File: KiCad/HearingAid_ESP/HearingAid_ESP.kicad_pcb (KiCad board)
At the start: 2 copper layers, 69.2 x 22.1 mm, 63 parts, among them J1 12402012E212A, Q1 PMOS, Q2 FS8205A, U1 AP2112K-3.3, U2 MAX98357A, U3 TP4056, U4 DW01A, U5 MAX98357A, U8 ESP32-S3

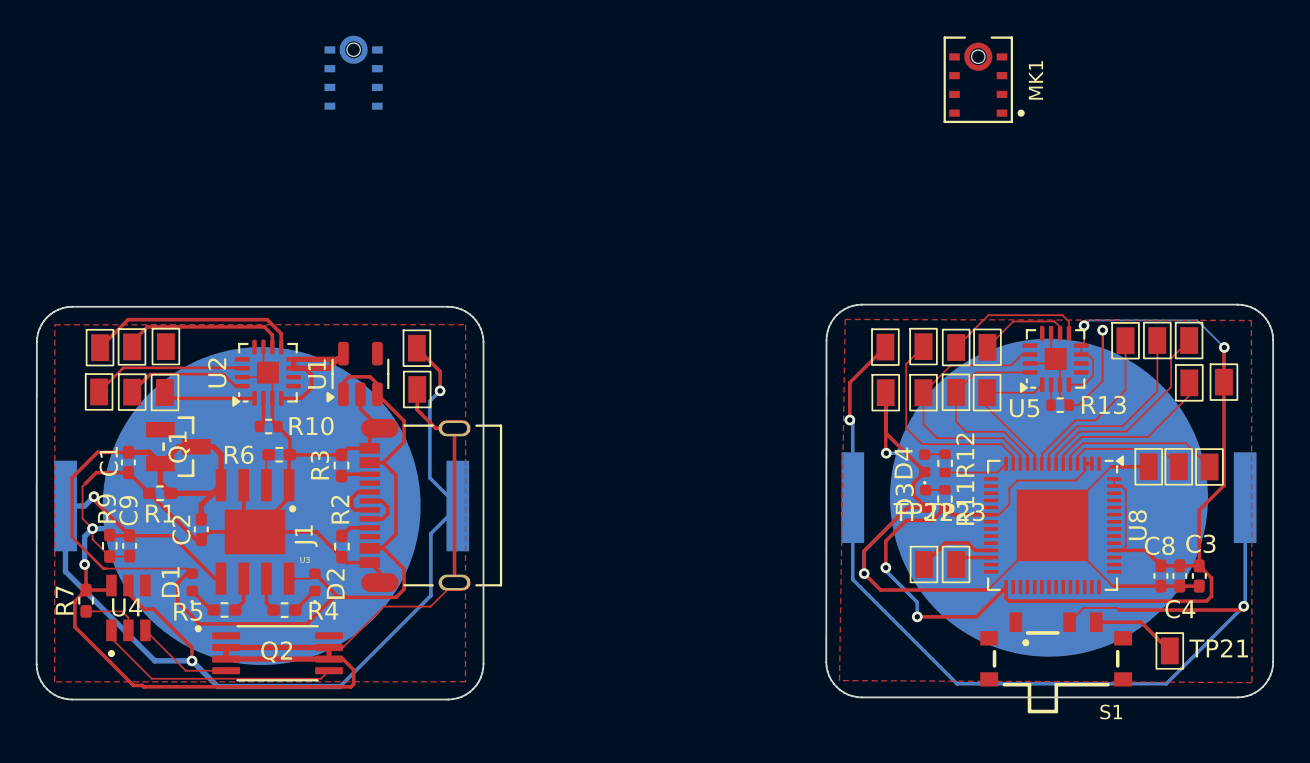
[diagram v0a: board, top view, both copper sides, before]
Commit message: Updating files
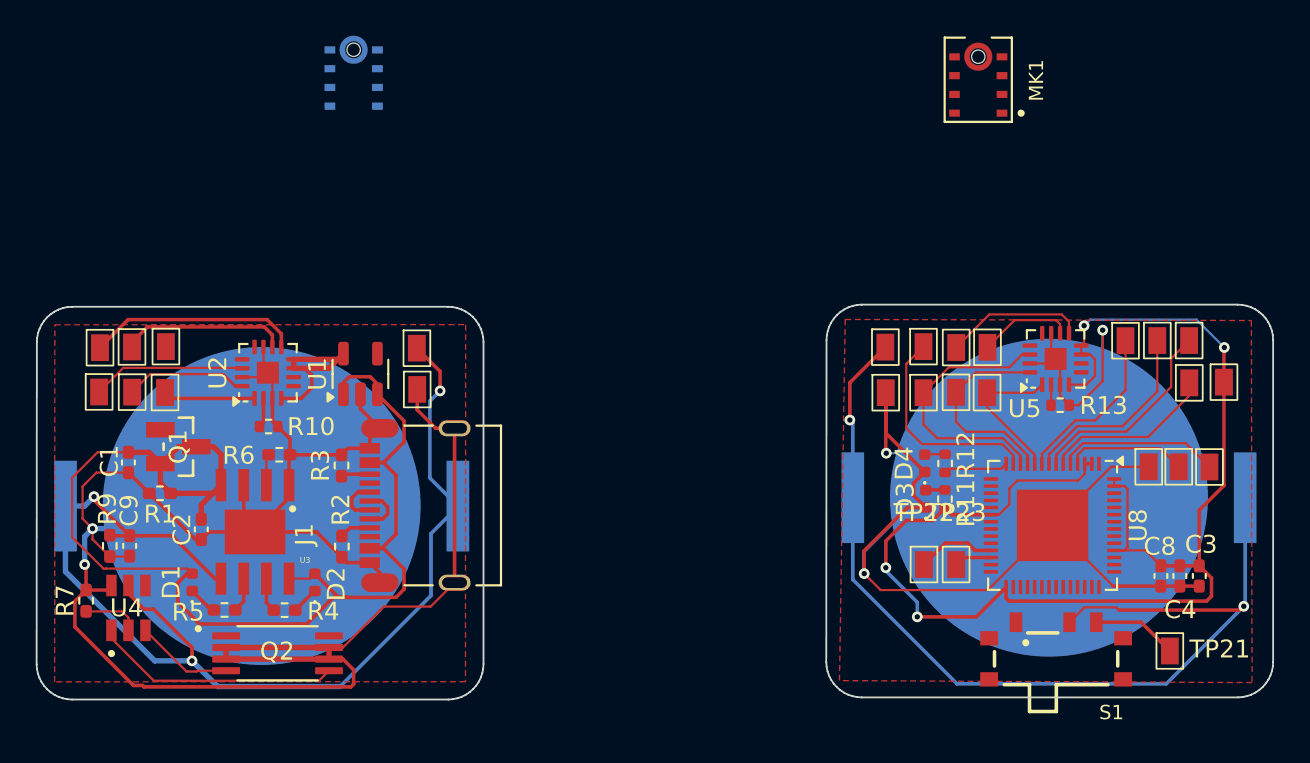
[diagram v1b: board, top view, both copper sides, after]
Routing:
- net VDD_ESP: track 86.2 -> 86.8 mm
